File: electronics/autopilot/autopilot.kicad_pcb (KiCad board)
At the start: 2 copper layers, 70.4 x 68.8 mm, 30 parts, among them J1 SERVO, J10 MPPT_I2C, J11 Debug, J12 5V IN, J13 Vbatt, J2 SERVO, J3 SERVO, J4 SERVO, J5 ESC, J6 GSM_MODULE, J7 IBUS, J8 5V IN, J9 IMU, SW1 ARM, U1 Pico, U2 SIM28ML, U3 NRF24L01_Breakout, U4 74HC244

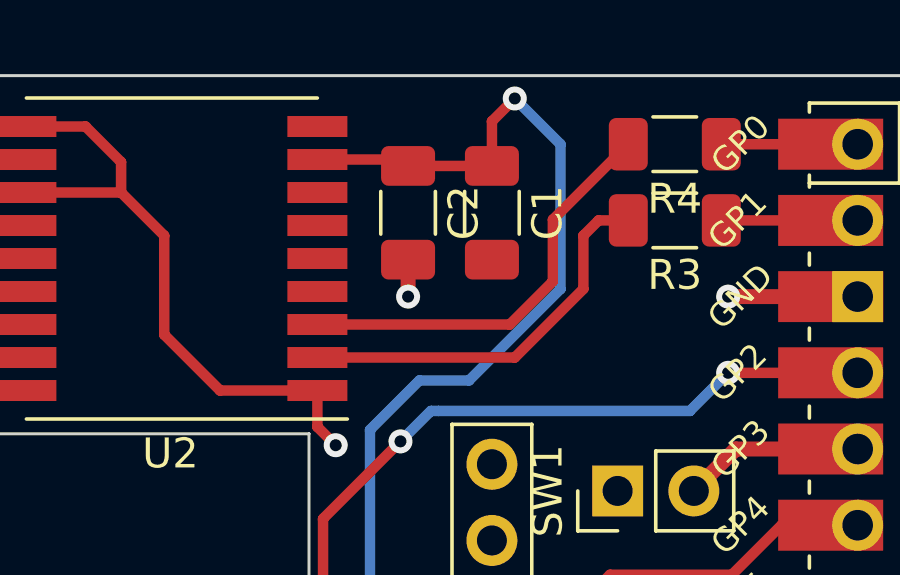
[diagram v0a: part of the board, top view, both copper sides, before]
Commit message: 3d renders of electronics
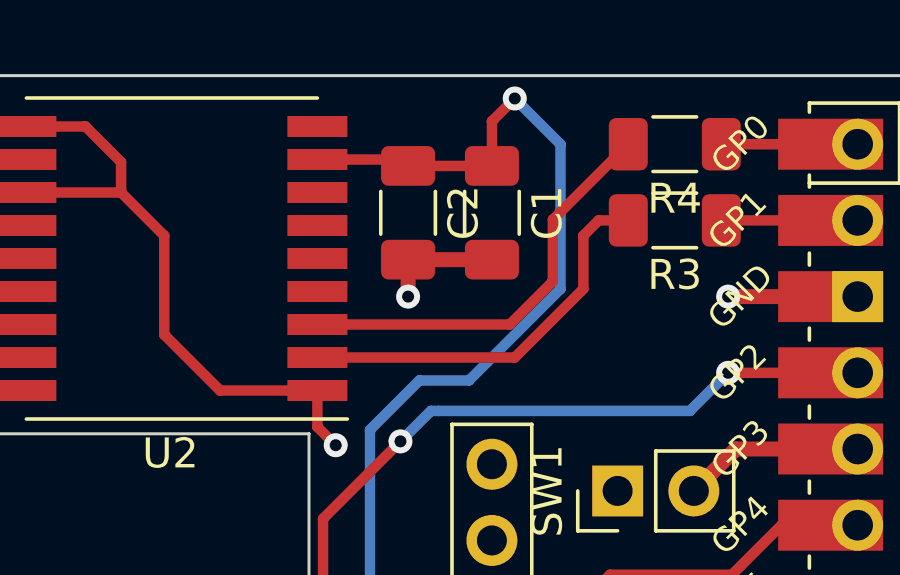
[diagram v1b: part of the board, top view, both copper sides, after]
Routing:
- net GND: track 100.2 -> 103.0 mm
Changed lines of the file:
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@@
   (segment (start 106.004 78.445) (end 107.442 79.883) (width 0.35) (layer "F.Cu") (net 3))
   (segment (start 102.846 76.245) (end 104.82 76.245) (width 0.35) (layer "F.Cu") (net 3))
+  (segment (start 115.57 80.6835) (end 118.364 80.6835) (width 0.5) (layer "F.Cu") (net 3))
   (segment (start 115.57 80.6835) (end 115.57 81.915) (width 0.5) (layer "F.Cu") (net 3))
   (segment (start 137.922 138.049) (end 137.354 138.617) (width 0.35) (layer "F.Cu") (net 3))
